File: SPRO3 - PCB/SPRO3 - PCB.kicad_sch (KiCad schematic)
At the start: 43 parts, among them J1 Power Input, J10 Conn_01x03_Pin, J11 Conn_01x03_Pin, J12 Conn_01x03_Pin, J13 Conn_01x03_Pin, J14 Conn_01x03_Pin, J15 Conn_01x03_Pin, J16 Spare I2C PINS, J2 2nd PCB, J3 Servo Motor, J4 L298N Module, J5 Gate Sensor, J6 Magnometer, J7 GPS Module, J8 Conn_01x03_Pin, J9 Conn_01x03_Pin, SW1 SW_SPDT, U1 ${SIM.PARAMS}, U2 CD4051B

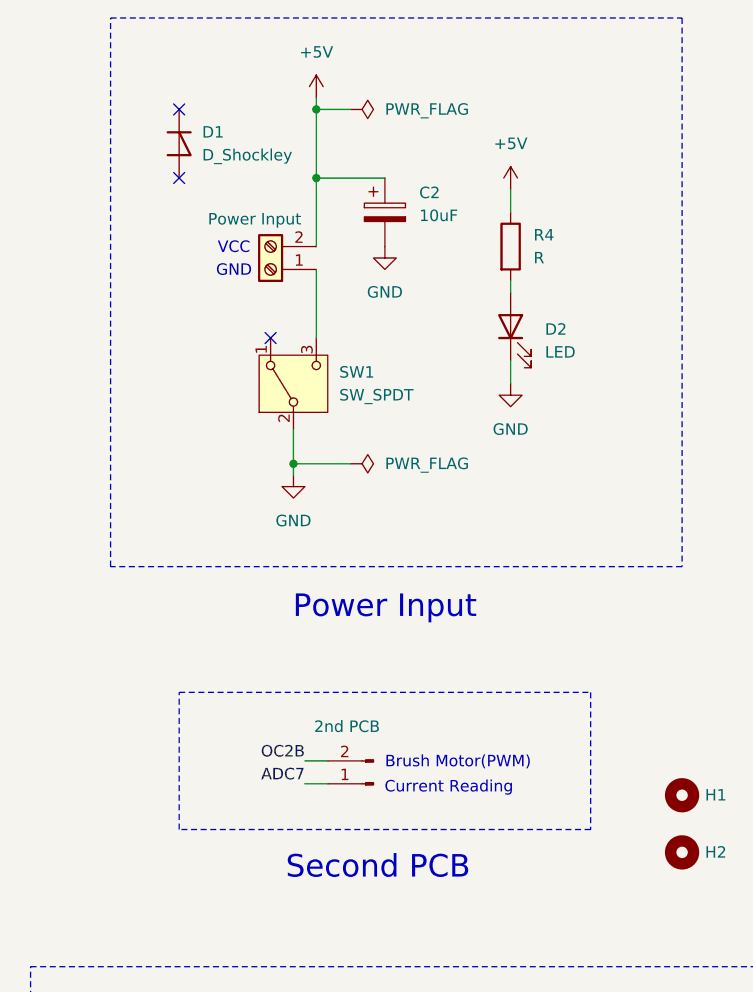
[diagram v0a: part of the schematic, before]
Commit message: finished the PCB board designs
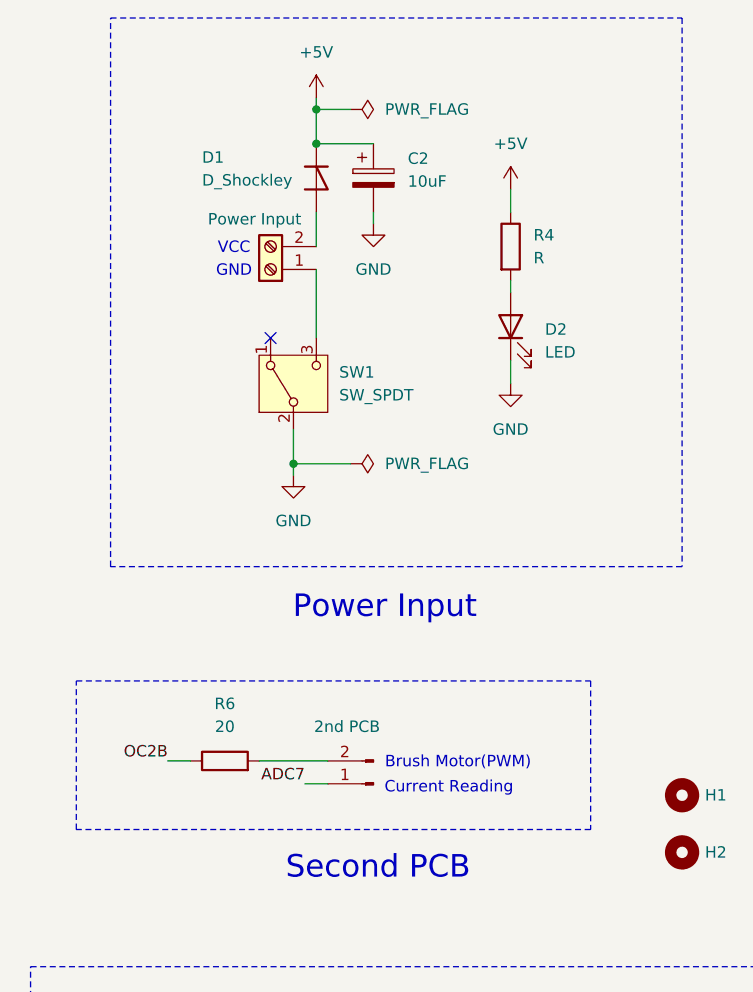
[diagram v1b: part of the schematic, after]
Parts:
- added R6: 20, Resistor_THT:R_Axial_DIN0207_L6.3mm_D2.5mm_P7.62mm_Horizontal, symbol Device:R
- H1, H2, H3, H4: footprint MountingHole:MountingHole_4.3mm_M4 -> MountingHole:MountingHole_3.2mm_M3
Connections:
- net +5V: now also D1.1 (K); no longer J1.2 (Pin_2)
- net OC2B: now also R6.1; no longer J2.2 (Pin_2)
- net at D1.2 (A): now also J1.2 (Pin_2)
- new net: J2.2 (Pin_2), R6.2
- no-connect marks 16 -> 14
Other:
- moved on the sheet: C2, D1
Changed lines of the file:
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@@
 	)
 	(junction
-		(at 49.53 33.02)
-		(diameter 0)
-		(color 0 0 0 0)
-	)
-	(junction
 		(at 233.68 62.23)
 		(diameter 0)
@@
 	)
 	(junction
-		(at 49.53 25.4)
-		(diameter 0)
-		(color 0 0 0 0)
-	)
-	(junction
 		(at 60.96 144.78)
 		(diameter 0)
@@
 	)
 	(junction
+		(at 49.53 25.4)
+		(diameter 0)
+		(color 0 0 0 0)
+	)
+	(junction
 		(at 43.18 132.08)
 		(diameter 0)
@@
 	)
 	(junction
+		(at 49.53 29.21)
+		(diameter 0)
+		(color 0 0 0 0)
+	)
+	(junction
 		(at 68.58 166.37)
 		(diameter 0)
@@
 	)
 	(no_connect
-		(at 34.29 33.02)
-	)
-	(no_connect
 		(at 135.89 80.01)
 	)
@@
 	)
 	(no_connect
-		(at 34.29 25.4)
-	)
-	(no_connect
 		(at 146.05 39.37)
 	)
@@
 	(wire
 		(pts
-			(xy 49.53 33.02) (xy 49.53 40.64)
-		)
-		(stroke
-			(width 0)
-			(type default)
-		)
-	)
-	(wire
-		(pts
 			(xy 238.76 50.8) (xy 241.3 50.8)
 		)
@@
 	(wire
 		(pts
+			(xy 33.02 97.79) (xy 35.56 97.79)
+		)
+		(stroke
+			(width 0)
+			(type default)
+		)
+	)
+	(wire
+		(pts
 			(xy 134.62 165.1) (xy 137.16 165.1)
 		)
@@
 	(wire
 		(pts
+			(xy 43.18 97.79) (xy 50.8 97.79)
+		)
+		(stroke
+			(width 0)
+			(type default)
+		)
+	)
+	(wire
+		(pts
 			(xy 38.1 153.67) (xy 38.1 160.02)
 		)
@@
 	(wire
 		(pts
+			(xy 55.88 36.83) (xy 55.88 38.1)
+		)
+		(stroke
+			(width 0)
+			(type default)
+		)
+	)
+	(wire
+		(pts
 			(xy 116.84 52.07) (xy 120.65 52.07)
 		)
@@
 	(wire
 		(pts
+			(xy 49.53 29.21) (xy 55.88 29.21)
+		)
+		(stroke
+			(width 0)
+			(type default)
+		)
+	)
+	(wire
+		(pts
 			(xy 233.68 62.23) (xy 241.3 62.23)
 		)
@@
 	(wire
 		(pts
-			(xy 49.53 25.4) (xy 49.53 33.02)
-		)
-		(stroke
-			(width 0)
-			(type default)
-		)
-	)
-	(wire
-		(pts
 			(xy 190.5 134.62) (xy 198.12 134.62)
 		)
@@
 	(wire
 		(pts
-			(xy 57.15 33.02) (xy 49.53 33.02)
+			(xy 46.99 60.96) (xy 46.99 64.77)
 		)
 		(stroke
@@
 	(wire
 		(pts
-			(xy 46.99 60.96) (xy 46.99 64.77)
+			(xy 207.01 40.64) (xy 207.01 43.18)
 		)
 		(stroke
@@
 	(wire
 		(pts
-			(xy 207.01 40.64) (xy 207.01 43.18)
+			(xy 49.53 135.89) (xy 43.18 135.89)
 		)
 		(stroke
@@
 	(wire
 		(pts
-			(xy 49.53 135.89) (xy 43.18 135.89)
+			(xy 229.87 68.58) (xy 229.87 74.93)
 		)
 		(stroke
@@
 	(wire
 		(pts
-			(xy 229.87 68.58) (xy 229.87 74.93)
+			(xy 134.62 162.56) (xy 137.16 162.56)
 		)
 		(stroke
@@
 	(wire
 		(pts
-			(xy 134.62 162.56) (xy 137.16 162.56)
+			(xy 128.27 132.08) (xy 139.7 132.08)
 		)
 		(stroke
@@
 	(wire
 		(pts
-			(xy 128.27 132.08) (xy 139.7 132.08)
+			(xy 48.26 100.33) (xy 50.8 100.33)
 		)
 		(stroke
@@
 	(wire
 		(pts
-			(xy 48.26 100.33) (xy 50.8 100.33)
+			(xy 49.53 36.83) (xy 49.53 40.64)
 		)
 		(stroke
@@
 	(wire
 		(pts
-			(xy 233.68 71.12) (xy 241.3 71.12)
+			(xy 49.53 25.4) (xy 49.53 29.21)
 		)
 		(stroke
@@
 	(wire
 		(pts
-			(xy 48.26 97.79) (xy 50.8 97.79)
+			(xy 233.68 71.12) (xy 241.3 71.12)
 		)
 		(stroke
@@
 	)
 	(rectangle
-		(start 34.29 90.17)
+		(start 22.86 88.9)
 		(end 80.01 105.41)
 		(stroke
@@
 	)
 	(label "OC2B"
-		(at 48.26 97.79 180)
+		(at 33.02 97.79 180)
 		(fields_autoplaced yes)
 		(effects
@@
 		)
 	)
+	(netclass_flag ""
+		(length 1)
+		(shape dot)
+		(at 49.53 38.1 270)
+		(fields_autoplaced yes)
+		(effects
+			(font
+				(size 1.27 1.27)
+			)
+			(justify right bottom)
+		)
+		(property "Netclass" "Power"
+			(at 50.53 37.4015 90)
+			(effects
+				(font
+					(size 1.27 1.27)
+					(italic yes)
+				)
+				(justify left)
+				(hide yes)
+			)
+		)
+	)
 	(symbol
 		(lib_id "power:GND")
@@
 	)
 	(symbol
+		(lib_id "Device:R")
+		(at 39.37 97.79 90)
+		(unit 1)
+		(exclude_from_sim no)
+		(in_bom yes)
+		(on_board yes)
+		(dnp no)
+		(fields_autoplaced yes)
+		(property "Reference" "R6"
+			(at 39.37 91.44 90)
+			(effects
+				(font
+					(size 1.27 1.27)
+				)
+			)
+		)
+		(property "Value" "20"
+			(at 39.37 93.98 90)
+			(effects
+				(font
+					(size 1.27 1.27)
+				)
+			)
+		)
+		(property "Footprint" "Resistor_THT:R_Axial_DIN0207_L6.3mm_D2.5mm_P7.62mm_Horizontal"
+			(at 39.37 99.568 90)
+			(effects
+				(font
+					(size 1.27 1.27)
+				)
+				(hide yes)
+			)
+		)
+		(property "Datasheet" "~"
+			(at 39.37 97.79 0)
+			(effects
+				(font
+					(size 1.27 1.27)
+				)
+				(hide yes)
+			)
+		)
+		(property "Description" "Resistor"
+			(at 39.37 97.79 0)
+			(effects
+				(font
+					(size 1.27 1.27)
+				)
+				(hide yes)
+			)
+		)
+		(pin "2"
+		)
+		(pin "1"
+		)
+		(instances
+			(project ""
+				(path "/53da7c59-d564-4ca1-aec6-a8473e4863ca"
+					(reference "R6")
+					(unit 1)
+				)
+			)
+		)
+	)
+	(symbol
 		(lib_id "Connector:Conn_01x03_Pin")
 		(at 246.38 41.91 0)
@@
 			)
 		)
-		(property "Footprint" "MountingHole:MountingHole_4.3mm_M4"
+		(property "Footprint" "MountingHole:MountingHole_3.2mm_M3"
 			(at 100.33 107.95 0)
 			(effects
@@
 			)
 		)
-		(property "Footprint" "MountingHole:MountingHole_4.3mm_M4"
+		(property "Footprint" "MountingHole:MountingHole_3.2mm_M3"
 			(at 100.33 101.6 0)
 			(effects
@@
 	(symbol
 		(lib_id "Device:D_Shockley")
-		(at 34.29 29.21 270)
+		(at 49.53 33.02 270)
 		(unit 1)
 		(exclude_from_sim no)
@@
 		(on_board yes)
 		(dnp no)
-		(fields_autoplaced yes)
 		(property "Reference" "D1"
-			(at 36.83 27.9399 90)
+			(at 36.83 30.734 90)
 			(effects
 				(font
@@
 		)
 		(property "Value" "D_Shockley"
-			(at 36.83 30.4799 90)
+			(at 36.83 33.274 90)
 			(effects
 				(font
@@
 		)
 		(property "Footprint" "Diode_THT:D_DO-41_SOD81_P10.16mm_Horizontal"
-			(at 34.29 29.21 0)
+			(at 49.53 33.02 0)
 			(effects
 				(font
@@
 		)
 		(property "Datasheet" "~"
-			(at 34.29 29.21 0)
+			(at 49.53 33.02 0)
 			(effects
 				(font
@@
 		)
 		(property "Description" "Shockley (PNPN) diode"
-			(at 34.29 29.21 0)
+			(at 49.53 33.02 0)
 			(effects
 				(font
@@
 	(symbol
 		(lib_id "power:GND")
-		(at 57.15 40.64 0)
+		(at 55.88 38.1 0)
 		(unit 1)
 		(exclude_from_sim no)
@@
 		(fields_autoplaced yes)
 		(property "Reference" "#PWR030"
-			(at 57.15 46.99 0)
+			(at 55.88 44.45 0)
 			(effects
 				(font
@@
 		)
 		(property "Value" "GND"
-			(at 57.15 45.72 0)
+			(at 55.88 43.18 0)
 			(effects
 				(font
@@
 		)
 		(property "Footprint" ""
-			(at 57.15 40.64 0)
+			(at 55.88 38.1 0)
 			(effects
 				(font
@@
 		)
 		(property "Datasheet" ""
-			(at 57.15 40.64 0)
+			(at 55.88 38.1 0)
 			(effects
 				(font
@@
 		)
 		(property "Description" "Power symbol creates a global label with name \"GND\" , ground"
-			(at 57.15 40.64 0)
+			(at 55.88 38.1 0)
 			(effects
 				(font
@@
 	(symbol
 		(lib_id "Device:C_Polarized")
-		(at 57.15 36.83 0)
+		(at 55.88 33.02 0)
 		(unit 1)
 		(exclude_from_sim no)
@@
 		(fields_autoplaced yes)
 		(property "Reference" "C2"
-			(at 60.96 34.6709 0)
+			(at 59.69 30.8609 0)
 			(effects
 				(font
@@
 		)
 		(property "Value" "10uF"
-			(at 60.96 37.2109 0)
+			(at 59.69 33.4009 0)
 			(effects
 				(font
@@
 		)
 		(property "Footprint" "Capacitor_THT:CP_Radial_D5.0mm_P2.50mm"
-			(at 58.1152 40.64 0)
+			(at 56.8452 36.83 0)
 			(effects
 				(font
@@
 		)
 		(property "Datasheet" "~"
-			(at 57.15 36.83 0)
+			(at 55.88 33.02 0)
 			(effects
 				(font
@@
 		)
 		(property "Description" "Polarized capacitor"
-			(at 57.15 36.83 0)
+			(at 55.88 33.02 0)
 			(effects
 				(font
@@
 			)
 		)
-		(property "Footprint" "MountingHole:MountingHole_4.3mm_M4"
+		(property "Footprint" "MountingHole:MountingHole_3.2mm_M3"
 			(at 90.17 101.6 0)
 			(effects
@@
 			)
 		)
-		(property "Footprint" "MountingHole:MountingHole_4.3mm_M4"
+		(property "Footprint" "MountingHole:MountingHole_3.2mm_M3"
 			(at 90.17 107.95 0)
 			(effects
